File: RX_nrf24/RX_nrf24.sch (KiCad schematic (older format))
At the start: 46 parts, among them J1 USB_B_Micro, J2 Conn_01x03_Male, J3 Conn_Coaxial, J4 Conn_01x10_Male, J5 Conn_01x04_Female, J6 Conn_01x06_Male, J7 Conn_01x10_Male, J8 Conn_01x10_Male, SW1 SW_Push, U1 USBLC6-2SC6, U2 MCP1700-3302E_SOT23, U3 STM32F103C8Tx, U5 nRF24L01P, Y1 Crystal_GND24, Y2 Crystal_GND24

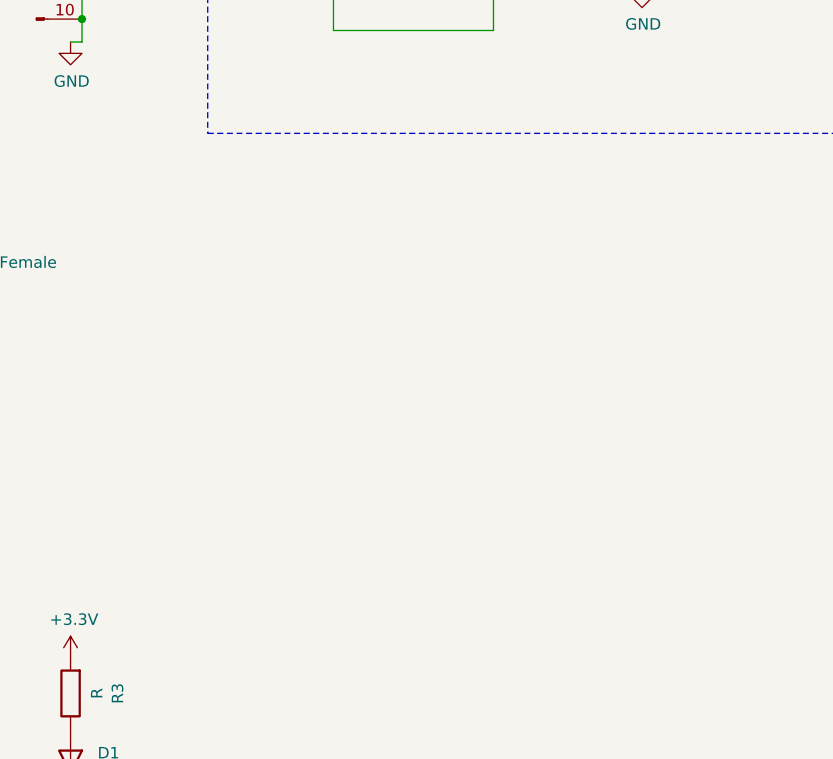
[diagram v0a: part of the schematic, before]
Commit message: add alot
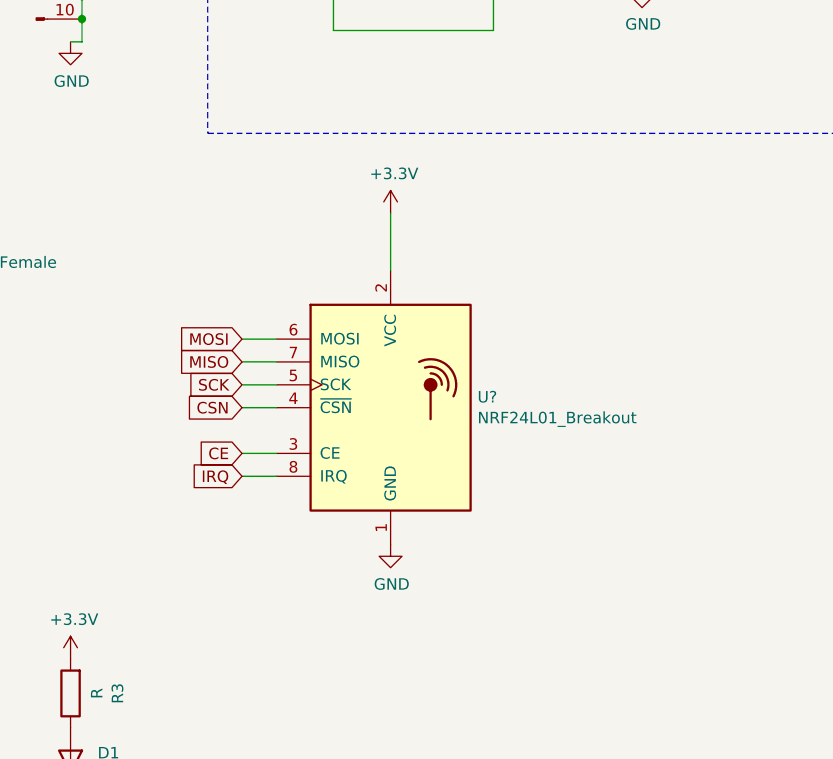
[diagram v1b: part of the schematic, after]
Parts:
- added U?: NRF24L01_Breakout, RF_Module:nRF24L01_Breakout, symbol RF:NRF24L01_Breakout
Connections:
- net +3V3: now also U?.2 (VCC)
- net CE: now also U?.3 (CE)
- net CSN: now also U?.4 (~CSN)
- net GND: now also U?.1 (GND)
- net IRQ: now also U?.8 (IRQ)
- net MISO: now also U?.7 (MISO)
- net MOSI: now also U?.6 (MOSI)
- net SCK: now also U?.5 (SCK)
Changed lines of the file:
@@
 	4900 1200 4500 1200
 Connection ~ 4500 1200
+$Comp
+L RF:NRF24L01_Breakout U?
+U 1 1 5F40A6BF
+P 7350 5200
+F 0 "U?" H 7730 5246 50  0000 L CNN
+F 1 "NRF24L01_Breakout" H 7730 5155 50  0000 L CNN
+F 2 "RF_Module:nRF24L01_Breakout" H 7500 5800 50  0001 L CIN
+F 3 "http://www.nordicsemi.com/eng/content/download/2730/34105/file/nRF24L01_Product_Specification_v2_0.pdf" H 7350 5100 50  0001 C CNN
+	1    7350 5200
+	1    0    0    -1
+$EndComp
+Wire Wire Line
+	7350 4600 7350 4350
+$Comp
+L power:+3.3V #PWR?
+U 1 1 5F40BF56
+P 7350 4350
+F 0 "#PWR?" H 7350 4200 50  0001 C CNN
+F 1 "+3.3V" H 7365 4523 50  0000 C CNN
+F 2 "" H 7350 4350 50  0001 C CNN
+F 3 "" H 7350 4350 50  0001 C CNN
+	1    7350 4350
+	1    0    0    -1
+$EndComp
+Text GLabel 6700 5400 0    50   Input ~ 0
+CE
+Text GLabel 6700 5200 0    50   Input ~ 0
+CSN
+Text GLabel 6700 5100 0    50   Input ~ 0
+SCK
+Text GLabel 6700 5000 0    50   Input ~ 0
+MISO
+Text GLabel 6700 4900 0    50   Input ~ 0
+MOSI
+Wire Wire Line
+	6700 5400 6850 5400
+Wire Wire Line
+	6700 5200 6850 5200
+Wire Wire Line
+	6850 5100 6700 5100
+Wire Wire Line
+	6700 5000 6850 5000
+Wire Wire Line
+	6700 4900 6850 4900
+Text GLabel 6700 5500 0    50   Input ~ 0
+IRQ
+Wire Wire Line
+	6700 5500 6850 5500
+$Comp
+L power:GND #PWR?
+U 1 1 5F451534
+P 7350 5800
+F 0 "#PWR?" H 7350 5550 50  0001 C CNN
+F 1 "GND" H 7355 5627 50  0000 C CNN
+F 2 "" H 7350 5800 50  0001 C CNN
+F 3 "" H 7350 5800 50  0001 C CNN
+	1    7350 5800
+	1    0    0    -1
+$EndComp
 $EndSCHEMATC
